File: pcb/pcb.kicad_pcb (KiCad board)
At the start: 2 copper layers, 52.5 x 28.7 mm, 30 parts, among them J4 Conn_02x05_Odd_Even, J5 RJ45_Amphenol_RJMG1BD3B8K1ANR, U1 ENC28J60x-SS, Y1 Crystal

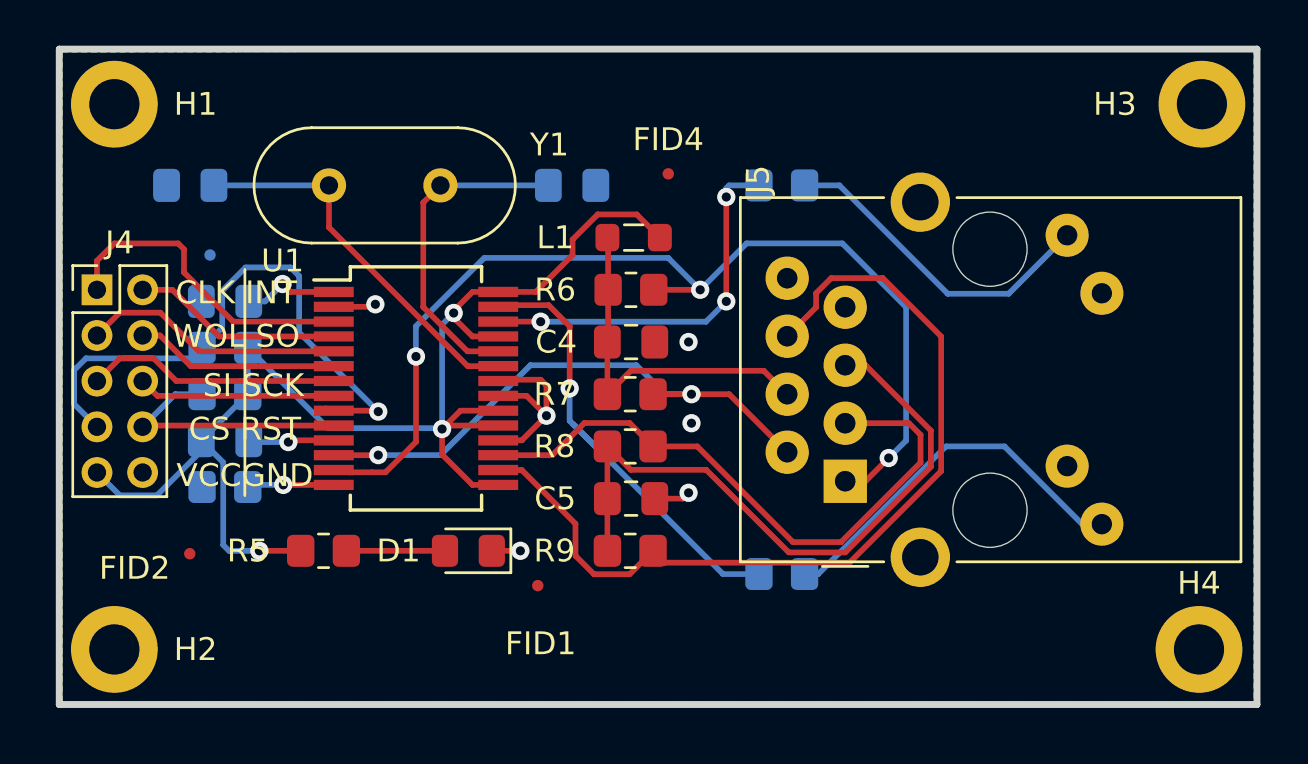
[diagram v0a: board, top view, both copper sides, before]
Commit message: Correcciones
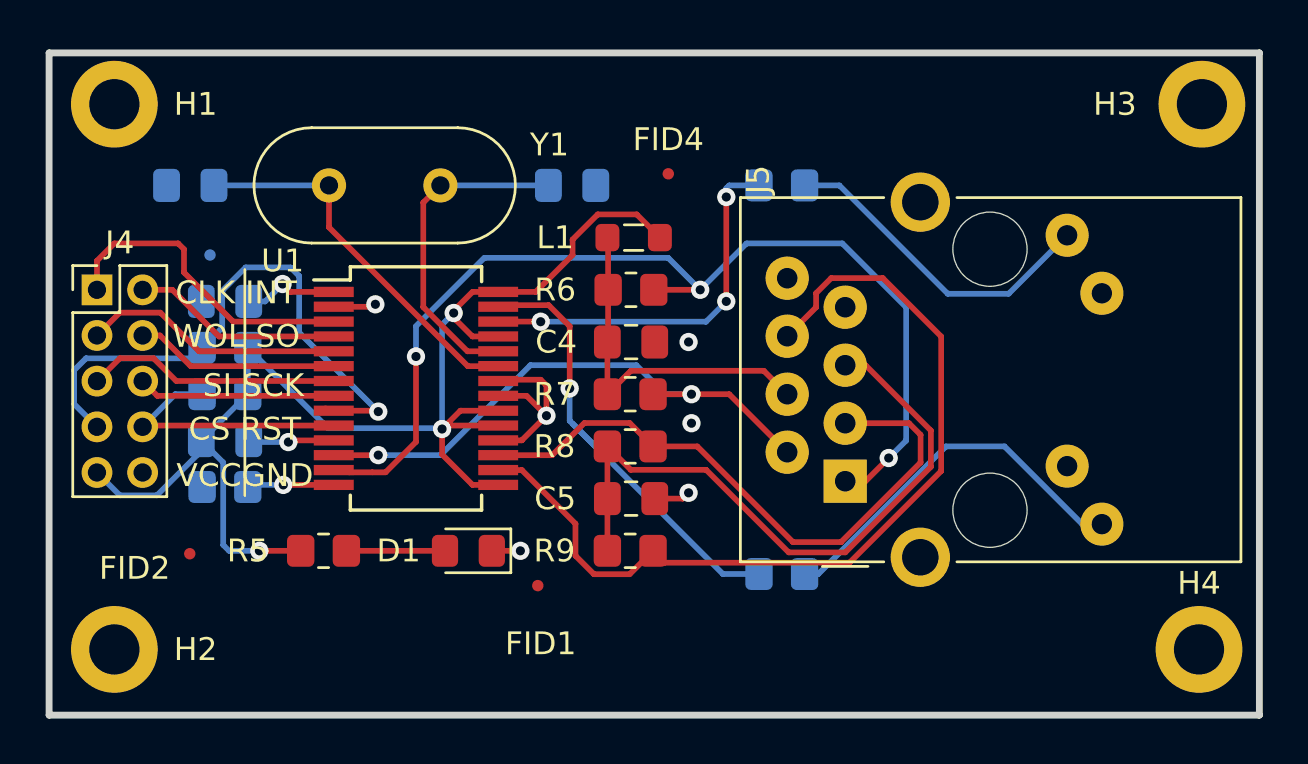
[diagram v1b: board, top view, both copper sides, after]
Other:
- board size 52.5 x 28.7 mm -> 53 x 29 mm
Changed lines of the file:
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@@
-      (effects (font (size 1 1) (thickness 0.15)))
-    )
-    (fp_text user %R (at 0.3 0) (layer F.Fab)
       (effects (font (size 1 1) (thickness 0.15)))
     )
     (fp_circle (center 0 0) (end 1.9 0) (layer Cmts.User) (width 0.15))
     (fp_circle (center 0 0) (end 2.15 0) (layer F.CrtYd) (width 0.05))
+    (fp_text user %R (at 0.3 0) (layer F.Fab)
+      (effects (font (size 1 1) (thickness 0.15)))
+    )
     (pad 1 thru_hole circle (at 0 0) (size 3.8 3.8) (drill 2.2) (layers *.Cu *.Mask))
   )
@@
       (effects (font (size 1 1) (thickness 0.15)))
     )
-    (fp_text user %R (at 0.3 0) (layer F.Fab)
-      (effects (font (size 1 1) (thickness 0.15)))
-    )
     (fp_circle (center 0 0) (end 1.9 0) (layer Cmts.User) (width 0.15))
     (fp_circle (center 0 0) (end 2.15 0) (layer F.CrtYd) (width 0.05))
+    (fp_text user %R (at 0.3 0) (layer F.Fab)
+      (effects (font (size 1 1) (thickness 0.15)))
+    )
     (pad 1 thru_hole circle (at 0 0) (size 3.8 3.8) (drill 2.2) (layers *.Cu *.Mask))
   )
@@
       (effects (font (size 1 1) (thickness 0.15)))
     )
-    (fp_text user %R (at 0.3 0) (layer F.Fab)
-      (effects (font (size 1 1) (thickness 0.15)))
-    )
     (fp_circle (center 0 0) (end 1.9 0) (layer Cmts.User) (width 0.15))
     (fp_circle (center 0 0) (end 2.15 0) (layer F.CrtYd) (width 0.05))
+    (fp_text user %R (at 0.3 0) (layer F.Fab)
+      (effects (font (size 1 1) (thickness 0.15)))
+    )
     (pad 1 thru_hole circle (at 0 0) (size 3.8 3.8) (drill 2.2) (layers *.Cu *.Mask))
   )
@@
       (effects (font (size 1 1) (thickness 0.15)))
     )
-    (fp_text user %R (at 0.3 0) (layer F.Fab)
-      (effects (font (size 1 1) (thickness 0.15)))
-    )
     (fp_circle (center 0 0) (end 1.9 0) (layer Cmts.User) (width 0.15))
     (fp_circle (center 0 0) (end 2.15 0) (layer F.CrtYd) (width 0.05))
+    (fp_text user %R (at 0.3 0) (layer F.Fab)
+      (effects (font (size 1 1) (thickness 0.15)))
+    )
     (pad 1 thru_hole circle (at 0 0) (size 3.8 3.8) (drill 2.2) (layers *.Cu *.Mask))
   )
@@
     (pad R1 thru_hole rect (at 0 0 90) (size 1.9 1.9) (drill 0.9) (layers *.Cu *.Mask)
       (net 20 "Net-(J5-PadR1)"))
-    (model ${KISYS3DMOD}/Connector_RJ.3dshapes/RJ45_Amphenol_RJMG1BD3B8K1ANR.wrl
-      (at (xyz 0 0 0))
-      (scale (xyz 1 1 1))
-      (rotate (xyz 0 0 0))
-    )
-    (model ${KIPRJMOD}/3dshapes/RJMG1BD3B8K1ANR.wrl
-      (at (xyz 0 0 0))
-      (scale (xyz 1 1 1))
-      (rotate (xyz 0 0 0))
-    )
     (model ${KIPRJMOD}/3dshapes/RJMG1BD3B8K1ANR.stp
       (at (xyz 0 0 0))
@@
     (effects (font (size 1 1) (thickness 0.15)))
   )
-  (gr_line (start 183.896 60.833) (end 183.896 89.535) (layer Edge.Cuts) (width 0.3))
-  (gr_line (start 131.445 60.833) (end 183.896 60.833) (layer Edge.Cuts) (width 0.3))
-  (gr_line (start 131.445 89.535) (end 131.445 60.833) (layer Edge.Cuts) (width 0.3))
-  (gr_line (start 131.445 89.535) (end 183.896 89.535) (layer Edge.Cuts) (width 0.3))
+  (gr_line (start 184 61) (end 184 90) (layer Edge.Cuts) (width 0.3))
+  (gr_line (start 131 61) (end 184 61) (layer Edge.Cuts) (width 0.3))
+  (gr_line (start 131 90) (end 131 61) (layer Edge.Cuts) (width 0.3))
+  (gr_line (start 131 90) (end 184 90) (layer Edge.Cuts) (width 0.3))
   (via (at 141.478 78.042) (size 0.8) (drill 0.4) (layers F.Cu B.Cu) (net 1))
   (segment (start 141.553 77.967) (end 141.478 78.042) (width 0.25) (layer F.Cu) (net 1))
@@
     (polygon
       (pts
-        (xy 183.769 89.535) (xy 131.572 89.408) (xy 131.572 60.96) (xy 183.769 60.833)
+        (xy 184 90) (xy 131 90) (xy 131 61) (xy 184 61)
       )
     )
@@
     (polygon
       (pts
-        (xy 183.769 89.408) (xy 131.572 89.408) (xy 131.572 60.96) (xy 183.769 60.833)
+        (xy 184 90) (xy 131 90) (xy 131 61) (xy 184 61)
       )
     )
